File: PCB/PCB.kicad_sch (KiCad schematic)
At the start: 212 parts, among them J1 Conn_01x04, J2 USB_C_Receptacle_USB2.0_16P, J3 Conn_01x05, U1 XC6206PxxxMR, U2 SRV05-4, U3 RP2040, U4 W25Q128JVS, Y1 Crystal_GND24

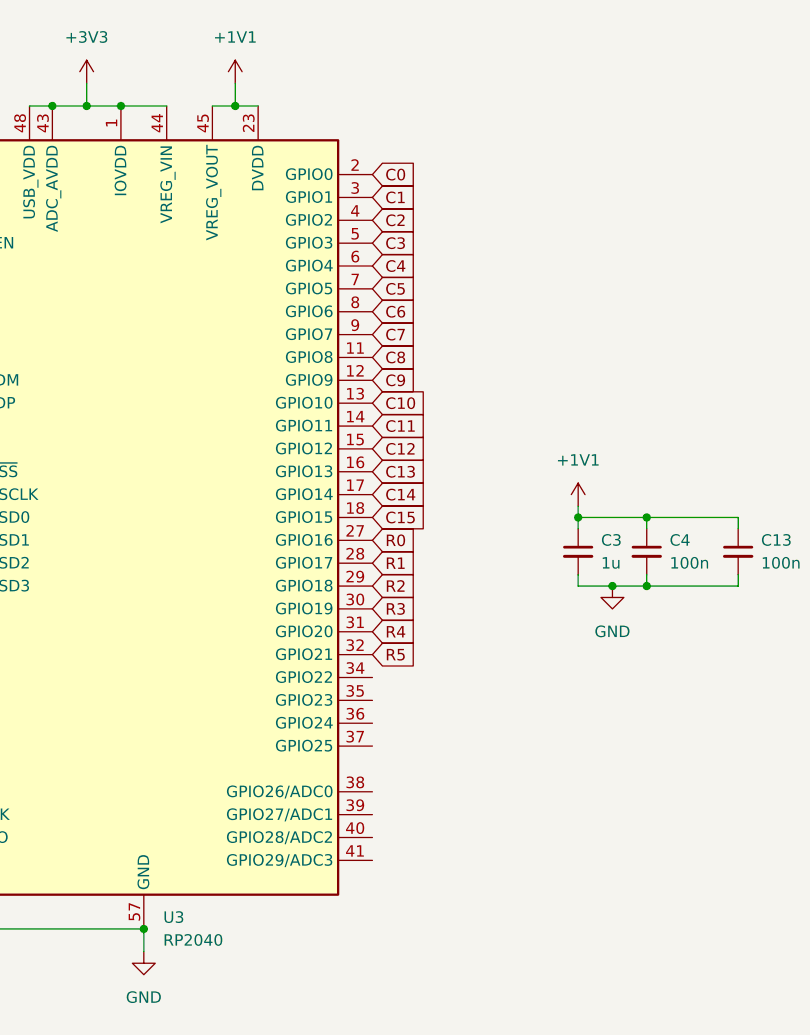
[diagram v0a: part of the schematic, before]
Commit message: keyboard matrix done
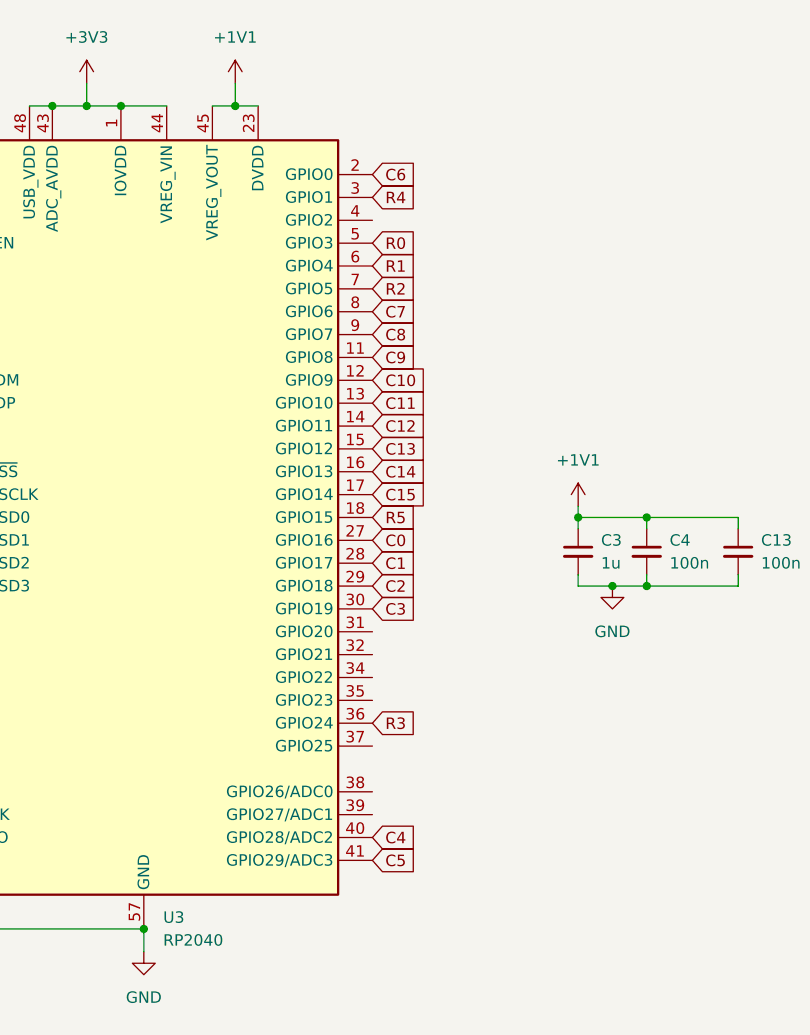
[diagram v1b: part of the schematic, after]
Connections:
- net C0: now also U3.27 (GPIO16); no longer U3.2 (GPIO0)
- net C1: now also U3.28 (GPIO17); no longer U3.3 (GPIO1)
- net C10: now also U3.12 (GPIO9); no longer U3.13 (GPIO10)
- net C11: now also U3.13 (GPIO10); no longer U3.14 (GPIO11)
- net C12: now also U3.14 (GPIO11); no longer U3.15 (GPIO12)
- net C13: now also U3.15 (GPIO12); no longer U3.16 (GPIO13)
- net C14: now also U3.16 (GPIO13); no longer U3.17 (GPIO14)
- net C15: now also U3.17 (GPIO14); no longer U3.18 (GPIO15)
- net C2: now also U3.29 (GPIO18); no longer U3.4 (GPIO2)
- net C3: now also U3.30 (GPIO19); no longer U3.5 (GPIO3)
- net C4: now also U3.40 (GPIO28/ADC2); no longer U3.6 (GPIO4)
- net C5: now also U3.41 (GPIO29/ADC3); no longer U3.7 (GPIO5)
- net C6: now also U3.2 (GPIO0); no longer U3.8 (GPIO6)
- net C7: now also U3.8 (GPIO6); no longer U3.9 (GPIO7)
- net C8: now also U3.9 (GPIO7); no longer U3.11 (GPIO8)
- net C9: now also U3.11 (GPIO8); no longer U3.12 (GPIO9)
- net R0: now also U3.5 (GPIO3); no longer U3.27 (GPIO16)
- net R1: now also U3.6 (GPIO4); no longer U3.28 (GPIO17)
- net R2: now also U3.7 (GPIO5); no longer U3.29 (GPIO18)
- net R3: now also U3.36 (GPIO24); no longer U3.30 (GPIO19)
- net R4: now also U3.3 (GPIO1); no longer U3.31 (GPIO20)
- net R5: now also U3.18 (GPIO15); no longer U3.32 (GPIO21)
